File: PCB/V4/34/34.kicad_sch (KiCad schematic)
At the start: 57 parts, among them J1 USB_C_Receptacle_USB2.0, J2 Conn_01x04, J3 AVR-ISP-6, J4 Conn_01x04, SW1 SW_Push, SW10 SW_Push, SW11 SW_Push, SW12 SW_Push, SW13 SW_Push, SW14 SW_Push, SW15 SW_Push, SW16 SW_Push, SW17 SW_Push, SW18 SW_Push, SW2 SW_Push, SW3 SW_Push, SW4 SW_Push, SW5 SW_Push, SW6 SW_Push, SW7 SW_Push, SW8 SW_Push, SW9 SW_Push, U1 ATmega32U4-AU, Y1 16MHz

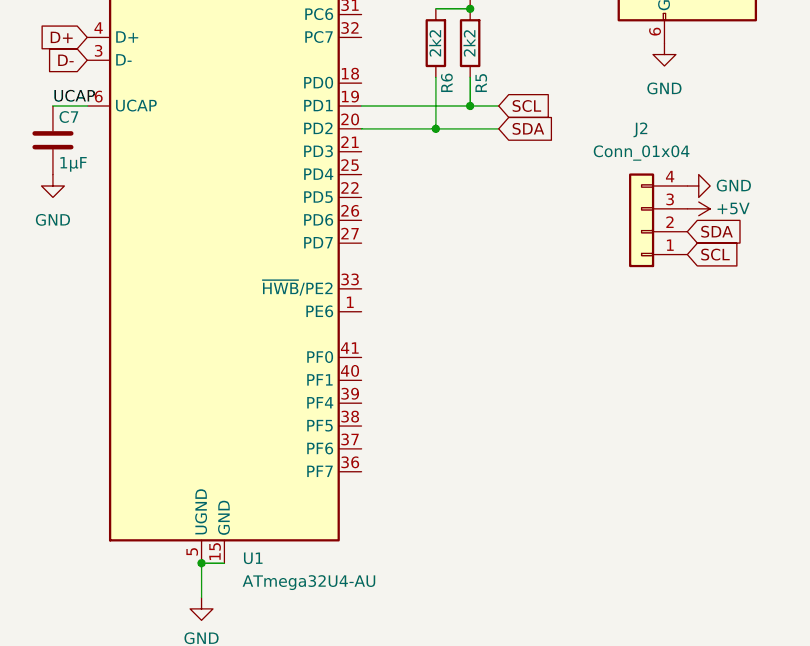
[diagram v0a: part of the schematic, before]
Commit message: right hand ready
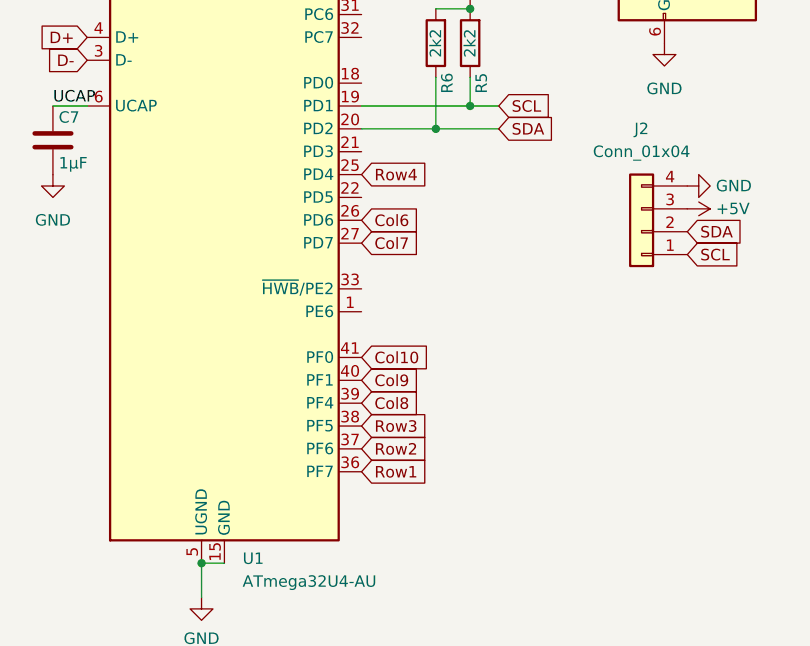
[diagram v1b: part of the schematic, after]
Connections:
- net Col10: now also U1.41 (PF0)
- net Col6: now also U1.26 (PD6)
- net Col7: now also U1.27 (PD7)
- net Col8: now also U1.39 (PF4)
- net Col9: now also U1.40 (PF1)
- net Row1: now also U1.36 (PF7)
- net Row2: now also U1.37 (PF6)
- net Row3: now also U1.38 (PF5)
- net Row4: now also U1.25 (PD4)
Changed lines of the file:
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@@
+    )
+  )
+  (global_label "Col9" (shape input) (at 123.19 119.38 0) (fields_autoplaced)
+    (effects (font (size 1.27 1.27)) (justify left))
+    (property "Intersheet References" "${INTERSHEET_REFS}" (id 0) (at 129.8969 119.4594 0)
+      (effects (font (size 1.27 1.27)) (justify left) hide)
     )
   )
@@
     )
   )
+  (global_label "Row3" (shape input) (at 123.19 124.46 0) (fields_autoplaced)
+    (effects (font (size 1.27 1.27)) (justify left))
+    (property "Intersheet References" "${INTERSHEET_REFS}" (id 0) (at 130.5621 124.3806 0)
+      (effects (font (size 1.27 1.27)) (justify left) hide)
+    )
+  )
   (global_label "Row1" (shape input) (at 195.58 37.465 180) (fields_autoplaced)
     (effects (font (size 1.27 1.27)) (justify right))
@@
     )
   )
+  (global_label "Row1" (shape input) (at 123.19 129.54 0) (fields_autoplaced)
+    (effects (font (size 1.27 1.27)) (justify left))
+    (property "Intersheet References" "${INTERSHEET_REFS}" (id 0) (at 130.5621 129.4606 0)
+      (effects (font (size 1.27 1.27)) (justify left) hide)
+    )
+  )
+  (global_label "Col7" (shape input) (at 123.19 104.14 0) (fields_autoplaced)
+    (effects (font (size 1.27 1.27)) (justify left))
+    (property "Intersheet References" "${INTERSHEET_REFS}" (id 0) (at 129.8969 104.0606 0)
+      (effects (font (size 1.27 1.27)) (justify left) hide)
+    )
+  )
   (global_label "D-" (shape input) (at 74.93 116.84 0) (fields_autoplaced)
     (effects (font (size 1.27 1.27)) (justify left))
     (property "Intersheet References" "${INTERSHEET_REFS}" (id 0) (at 80.1855 116.9194 0)
+      (effects (font (size 1.27 1.27)) (justify left) hide)
+    )
+  )
+  (global_label "Row2" (shape input) (at 123.19 127 0) (fields_autoplaced)
+    (effects (font (size 1.27 1.27)) (justify left))
+    (property "Intersheet References" "${INTERSHEET_REFS}" (id 0) (at 130.5621 126.9206 0)
       (effects (font (size 1.27 1.27)) (justify left) hide)
     )
@@
     )
   )
+  (global_label "Col8" (shape input) (at 123.19 121.92 0) (fields_autoplaced)
+    (effects (font (size 1.27 1.27)) (justify left))
+    (property "Intersheet References" "${INTERSHEET_REFS}" (id 0) (at 129.8969 121.8406 0)
+      (effects (font (size 1.27 1.27)) (justify left) hide)
+    )
+  )
+  (global_label "Col6" (shape input) (at 123.19 101.6 0) (fields_autoplaced)
+    (effects (font (size 1.27 1.27)) (justify left))
+    (property "Intersheet References" "${INTERSHEET_REFS}" (id 0) (at 129.8969 101.5206 0)
+      (effects (font (size 1.27 1.27)) (justify left) hide)
+    )
+  )
+  (global_label "Row4" (shape input) (at 123.19 96.52 0) (fields_autoplaced)
+    (effects (font (size 1.27 1.27)) (justify left))
+    (property "Intersheet References" "${INTERSHEET_REFS}" (id 0) (at 130.5621 96.4406 0)
+      (effects (font (size 1.27 1.27)) (justify left) hide)
+    )
+  )
   (global_label "Col8" (shape input) (at 238.76 22.225 90) (fields_autoplaced)
     (effects (font (size 1.27 1.27)) (justify left))
@@
       (effects (font (size 1.27 1.27)) (justify left) hide)
     )
+  )
+  (global_label "Col10" (shape input) (at 123.19 116.84 0) (fields_autoplaced)
+    (effects (font (size 1.27 1.27)) (justify left))
+    (property "Intersheet References" "${INTERSHEET_REFS}" (id 0) (at 131.1064 116.7606 0)
+      (effects (font (size 1.27 1.27)) (justify left) hide)
+    )
